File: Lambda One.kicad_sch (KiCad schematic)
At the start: 1 part, among them U1 W65C816SxP

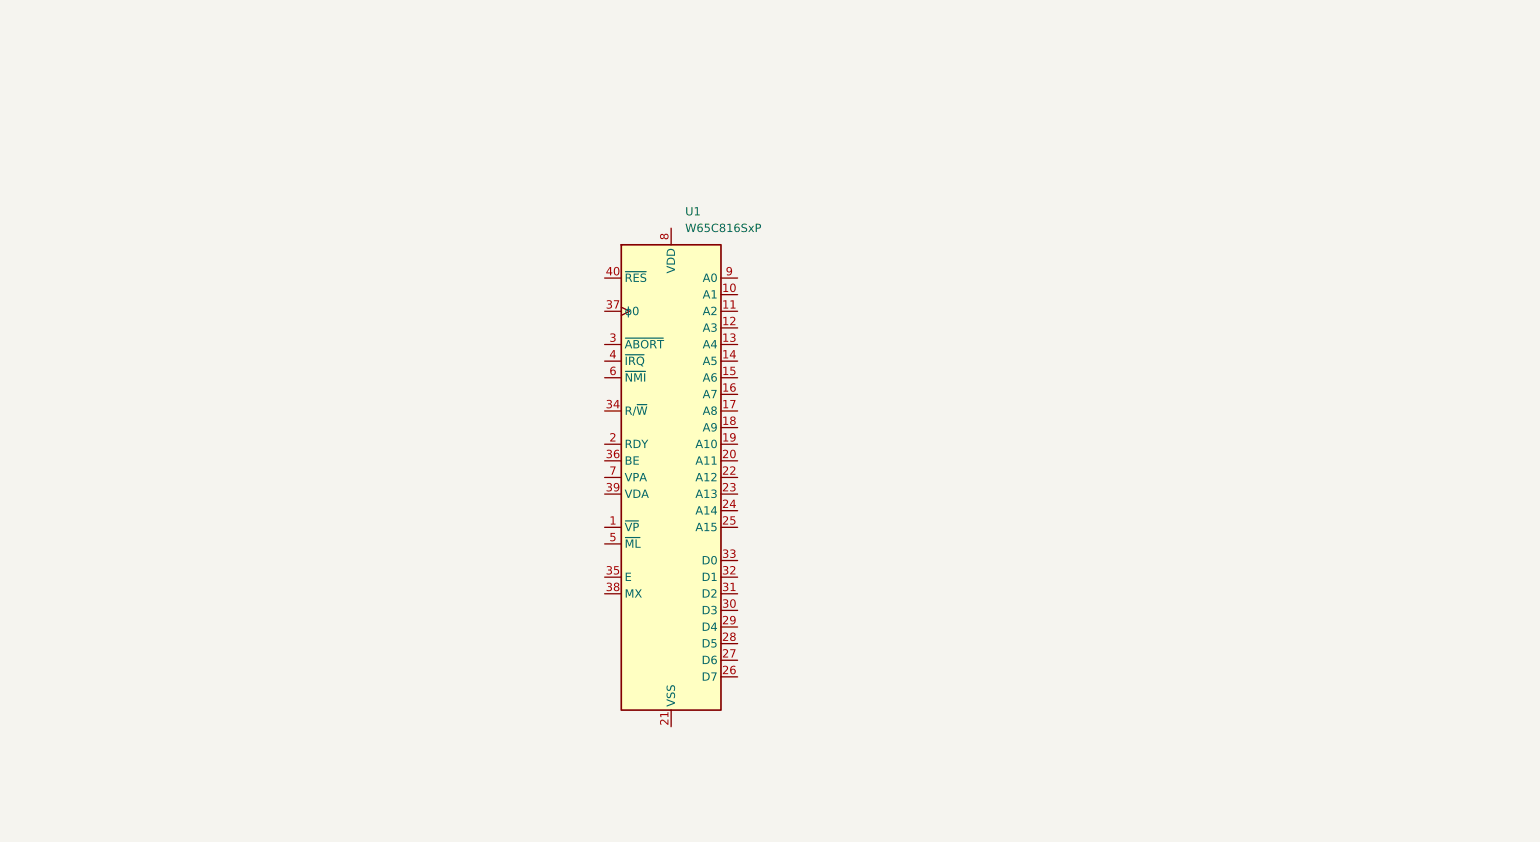
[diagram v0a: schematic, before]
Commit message: added ram and rom
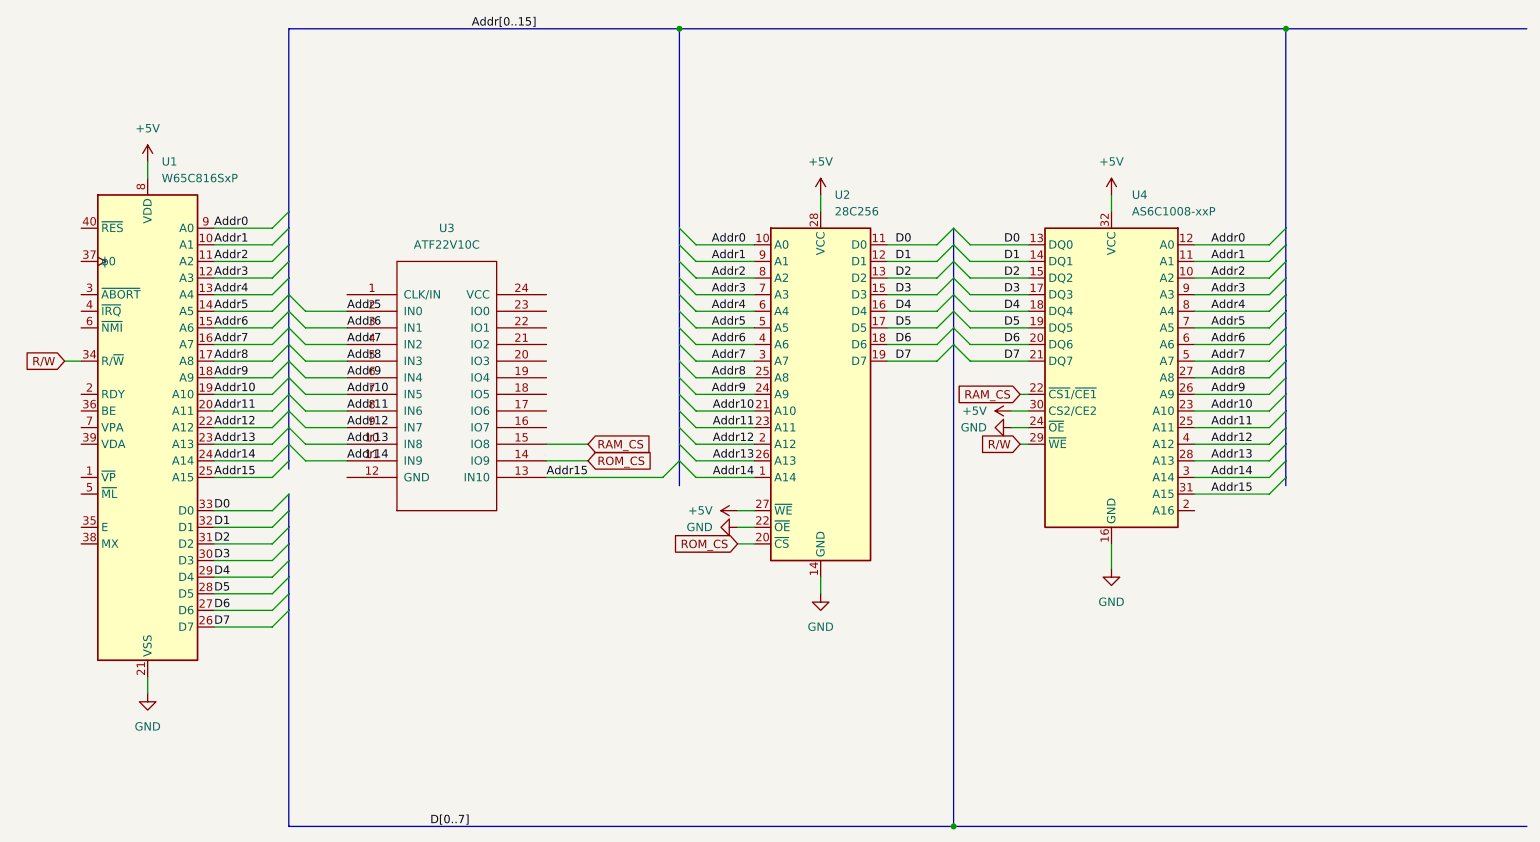
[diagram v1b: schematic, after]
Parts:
- added U2: 28C256, symbol Memory_EEPROM:28C256
- added U3: ATF22V10C, MODULE, symbol ATF22V10C:ATF22V10C
- added U4: AS6C1008-xxP, Package_DIP:DIP-32_W15.24mm, symbol Memory_RAM:AS6C1008-xxP
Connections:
- net Addr1: now reaches U1.10 (A1)
- net Addr1: now also U2.9 (A1), U4.11 (A1)
- net Addr2: now reaches U1.11 (A2)
- net Addr2: now also U2.8 (A2), U4.10 (A2)
- net Addr3: now reaches U1.12 (A3)
- net Addr3: now also U2.7 (A3), U4.9 (A3)
- net Addr4: now reaches U1.13 (A4)
- net Addr4: now also U2.6 (A4), U4.8 (A4)
- net Addr5: now reaches U1.14 (A5)
- net Addr5: now also U2.5 (A5), U3.2 (IN0), U4.7 (A5)
- net Addr6: now reaches U1.15 (A6)
- net Addr6: now also U2.4 (A6), U3.3 (IN1), U4.6 (A6)
- net Addr7: now reaches U1.16 (A7)
- net Addr7: now also U2.3 (A7), U3.4 (IN2), U4.5 (A7)
- net Addr8: now reaches U1.17 (A8)
- net Addr8: now also U2.25 (A8), U3.5 (IN3), U4.27 (A8)
- net Addr9: now reaches U1.18 (A9)
- net Addr9: now also U2.24 (A9), U3.6 (IN4), U4.26 (A9)
- net Addr10: now reaches U1.19 (A10)
- net Addr10: now also U2.21 (A10), U3.7 (IN5), U4.23 (A10)
- net Addr11: now reaches U1.20 (A11)
- net Addr11: now also U2.23 (A11), U3.8 (IN6), U4.25 (A11)
- net GND: now reaches U1.21 (VSS)
- net GND: now also U2.14 (GND), U2.22 (~{OE}), U4.16 (GND), U4.24 (~{OE})
- net Addr12: now reaches U1.22 (A12)
- net Addr12: now also U2.2 (A12), U3.9 (IN7), U4.4 (A12)
- net Addr13: now reaches U1.23 (A13)
- net Addr13: now also U2.26 (A13), U3.10 (IN8), U4.28 (A13)
- net Addr14: now reaches U1.24 (A14)
- net Addr14: now also U2.1 (A14), U3.11 (IN9), U4.3 (A14)
- net Addr15: now reaches U1.25 (A15)
- net Addr15: now also U3.13 (IN10), U4.31 (A15)
- net D7: now reaches U1.26 (D7)
- net D7: now also U2.19 (D7), U4.21 (DQ7)
- net D6: now reaches U1.27 (D6)
- net D6: now also U2.18 (D6), U4.20 (DQ6)
- net D5: now reaches U1.28 (D5)
- net D5: now also U2.17 (D5), U4.19 (DQ5)
- net D4: now reaches U1.29 (D4)
- net D4: now also U2.16 (D4), U4.18 (DQ4)
- net D3: now reaches U1.30 (D3)
- net D3: now also U2.15 (D3), U4.17 (DQ3)
- net D2: now reaches U1.31 (D2)
- net D2: now also U2.13 (D2), U4.15 (DQ2)
- net D1: now reaches U1.32 (D1)
- net D1: now also U2.12 (D1), U4.14 (DQ1)
- net D0: now reaches U1.33 (D0)
- net D0: now also U2.11 (D0), U4.13 (DQ0)
- net R/W: now reaches U1.34 (R/~{W})
- net R/W: now also U4.29 (~{WE})
- net +5V: now reaches U1.8 (VDD)
- net +5V: now also U2.27 (~{WE}), U2.28 (VCC), U4.30 (CS2/CE2), U4.32 (VCC)
- net Addr0: now reaches U1.9 (A0)
- net Addr0: now also U2.10 (A0), U4.12 (A0)
- new net RAM_CS: U3.15 (IO8), U4.22 (~{CS1}/~{CE1})
- new net ROM_CS: U2.20 (~{CS}), U3.14 (IO9)
